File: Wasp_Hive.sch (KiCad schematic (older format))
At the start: 124 parts, among them J0 WASP_OUT, J1 WASP_OUT, J10 WASP_OUT, J11 WASP_OUT, J12 WASP_OUT, J13 WASP_OUT, J14 WASP_OUT, J15 WASP_OUT, J16 FM_IN, J17 DENS_IN, J2 WASP_OUT, J3 WASP_OUT, J4 WASP_OUT, J5 WASP_OUT, J6 WASP_OUT, J7 WASP_OUT, J8 WASP_OUT, J9 WASP_OUT, Q1 MMBT3904, Q2 MMBT3904, U0 74HC245, U1 74HC245, U2 MCP6002-xP, U3 L78M05ABDT-TR, U4 MCP6002-xP, U5 TEENSY_3.2_MINIMAL

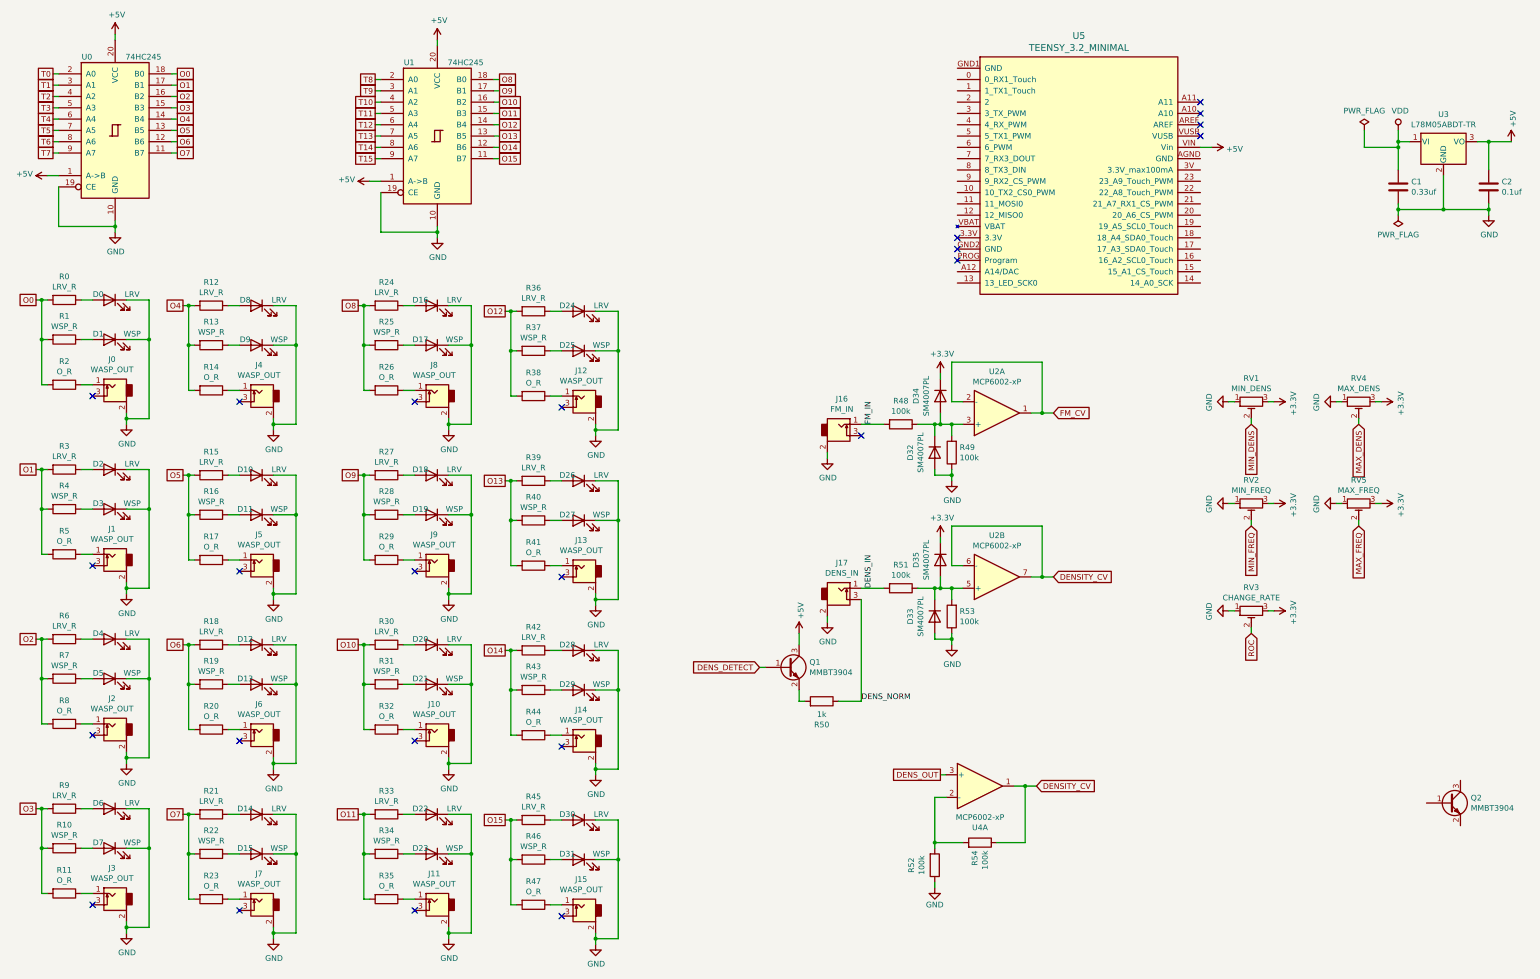
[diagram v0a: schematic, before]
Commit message: alterantive sketch
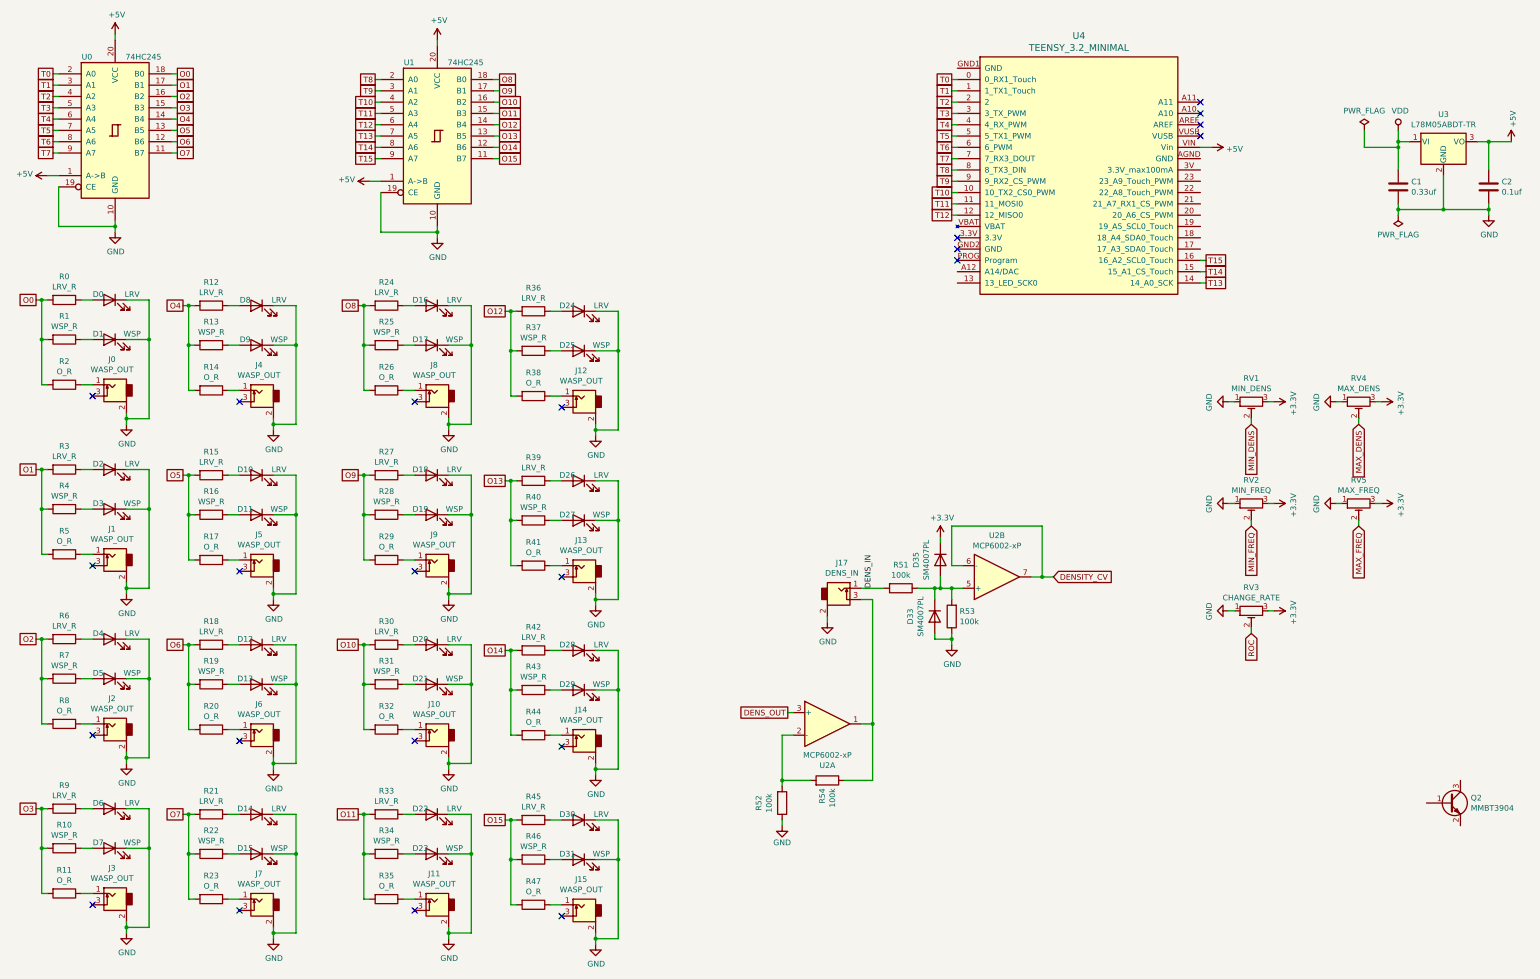
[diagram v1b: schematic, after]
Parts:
- removed D32, D34: SM4007PL, Diode_SMD:D_SOD-123, symbol Device:D
- removed J16: FM_IN, HammerheadAudio:EuroJack_MonoSW_THT_NOREF_Mask, symbol Connector:EuroJack_Mono_3.5mm_Switched
- removed Q1: MMBT3904, Package_TO_SOT_SMD:SOT-23, symbol Transistor_BJT:MMBT3904
- removed R48, R49: 100k, HammerheadAudio:R_THT_P7.62_Centered, symbol Device:R
- removed R50: 1k, HammerheadAudio:R_THT_P7.62_Centered, symbol Device:R
- removed unit 1 of U2
- renumbered U4 to U2, U5 to U4
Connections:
- net DENSITY_CV: no longer R54.1, U2.1
- net T0: now also U4.0 (0_RX1_Touch)
- net T1: now also U4.1 (1_TX1_Touch)
- net T10: now also U4.10 (10_TX2_CS0_PWM)
- net T11: now also U4.11 (11_MOSI0)
- net T12: now also U4.12 (12_MISO0)
- net T13: now also U4.14 (14_A0_SCK)
- net T14: now also U4.15 (15_A1_CS_Touch)
- net T15: now also U4.16 (16_A2_SCL0_Touch)
- net T2: now also U4.2
- net T3: now also U4.3 (3_TX_PWM)
- net T4: now also U4.4 (4_RX_PWM)
- net T5: now also U4.5 (5_TX1_PWM)
- net T6: now also U4.6 (6_PWM)
- net T7: now also U4.7 (7_RX3_DOUT)
- net T8: now also U4.8 (8_TX3_DIN)
- net T9: now also U4.9 (9_RX2_CS_PWM)
- net DENS_NORM: no longer names the net of J17.3
- net DENS_NORM: now also R54.1, U2.1
- no-connect marks 24 -> 23
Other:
- moved on the sheet: R52, R54, U2A
